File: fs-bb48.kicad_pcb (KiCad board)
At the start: 2 copper layers, 12 parts, among them P2 SWD, P3 PWR, P4 EXT, U1 MKL27Z256VFM4

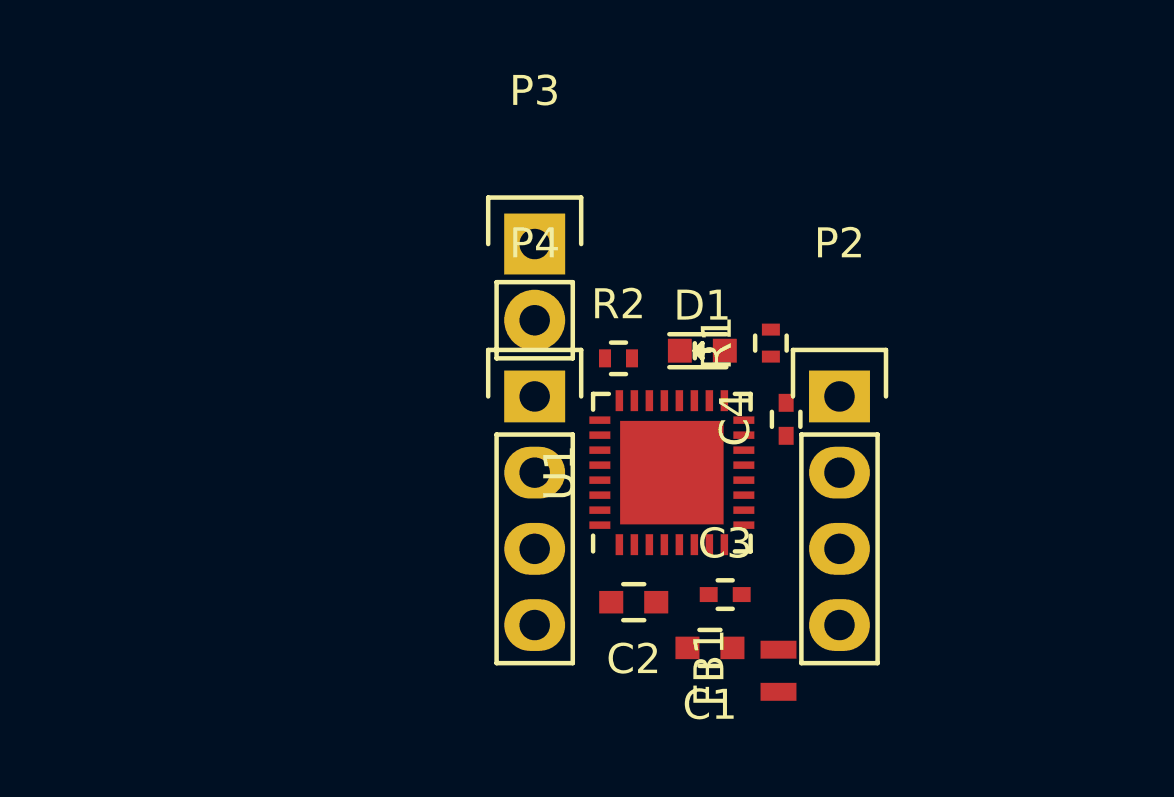
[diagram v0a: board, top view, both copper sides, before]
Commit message: add footprints
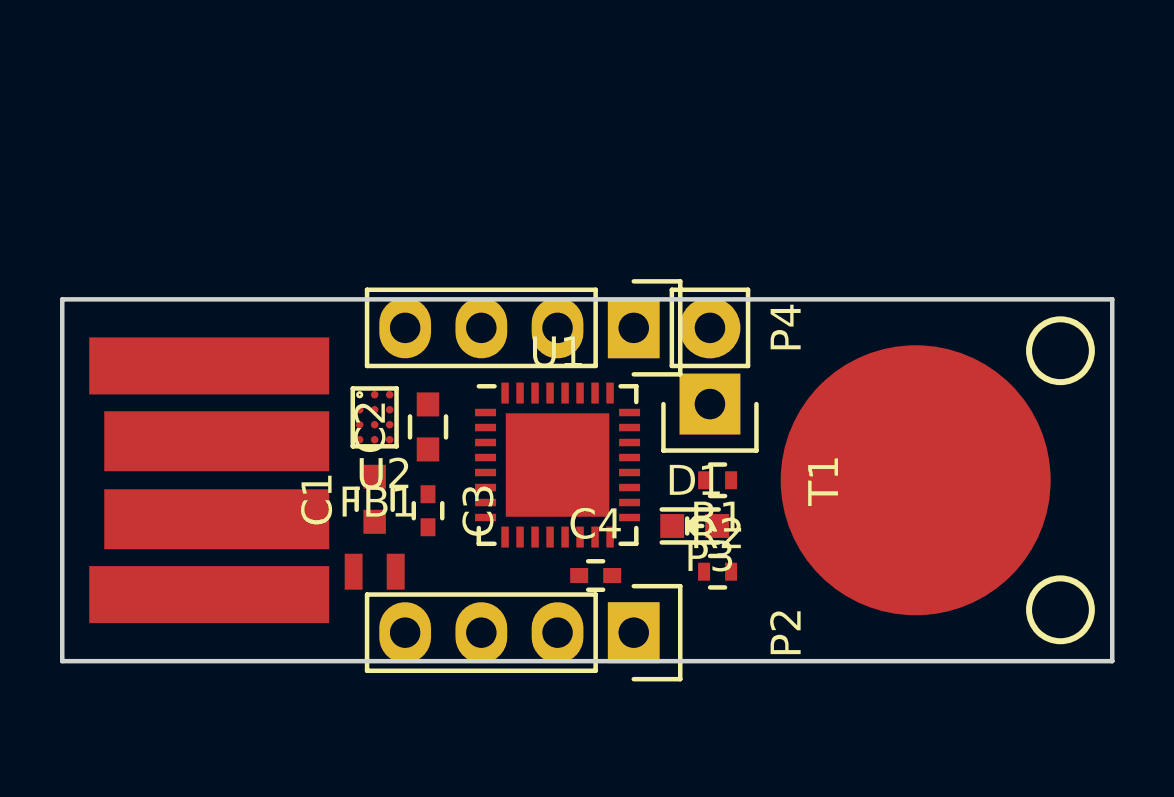
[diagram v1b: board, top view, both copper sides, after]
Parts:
- added P1: USB, fs-bb48:usb-PCB, F.Cu at (126.5, 106.9)
- added T1: TOUCH_PAD, fs-bb48:TOUCH_PAD_9mm, F.Cu at (154.9, 106.9)
- added U2: EMIF02-USB03F2, fs-bb48:BGA-11, F.Cu at (136.9, 105.3)
- moved FB1 13.9 mm to (136.9, 110.0), turned to 0 degrees
- moved C1 12.2 mm to (136.9, 107.6), turned to 90 degrees
- moved P2 10.4 mm to (145.5, 112.0), turned to 270 degrees
- moved C3 10.3 mm to (138.7, 108.0), turned to 270 degrees
- moved C2 9.01 mm to (138.7, 105.2), turned to 90 degrees
- moved C4 8.21 mm to (144.3, 110.1), turned to 0 degrees
- moved P3 7.91 mm to (148.1, 104.4), turned to 180 degrees
- moved R1 7.82 mm to (148.3, 110.0), turned to 0 degrees
- moved D1 5.85 mm to (147.6, 108.5)
- moved R2 5.24 mm to (148.3, 106.9), turned to 180 degrees
- moved P4 4.02 mm to (145.5, 101.9), turned to 270 degrees
- moved U1 3.82 mm to (143.0, 106.4), turned to 0 degrees
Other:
- board outline added: 35 x 12.1 mm
